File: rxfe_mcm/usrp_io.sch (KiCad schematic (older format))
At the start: 24 parts, among them J201 DB15, P201 CONN_02X10, U202 CONN_SMA, U203 74HC04_FULL, U204 CONN_SMA, U205 ADP7158, U206 CONN_SMA, U209 CONN_SMA

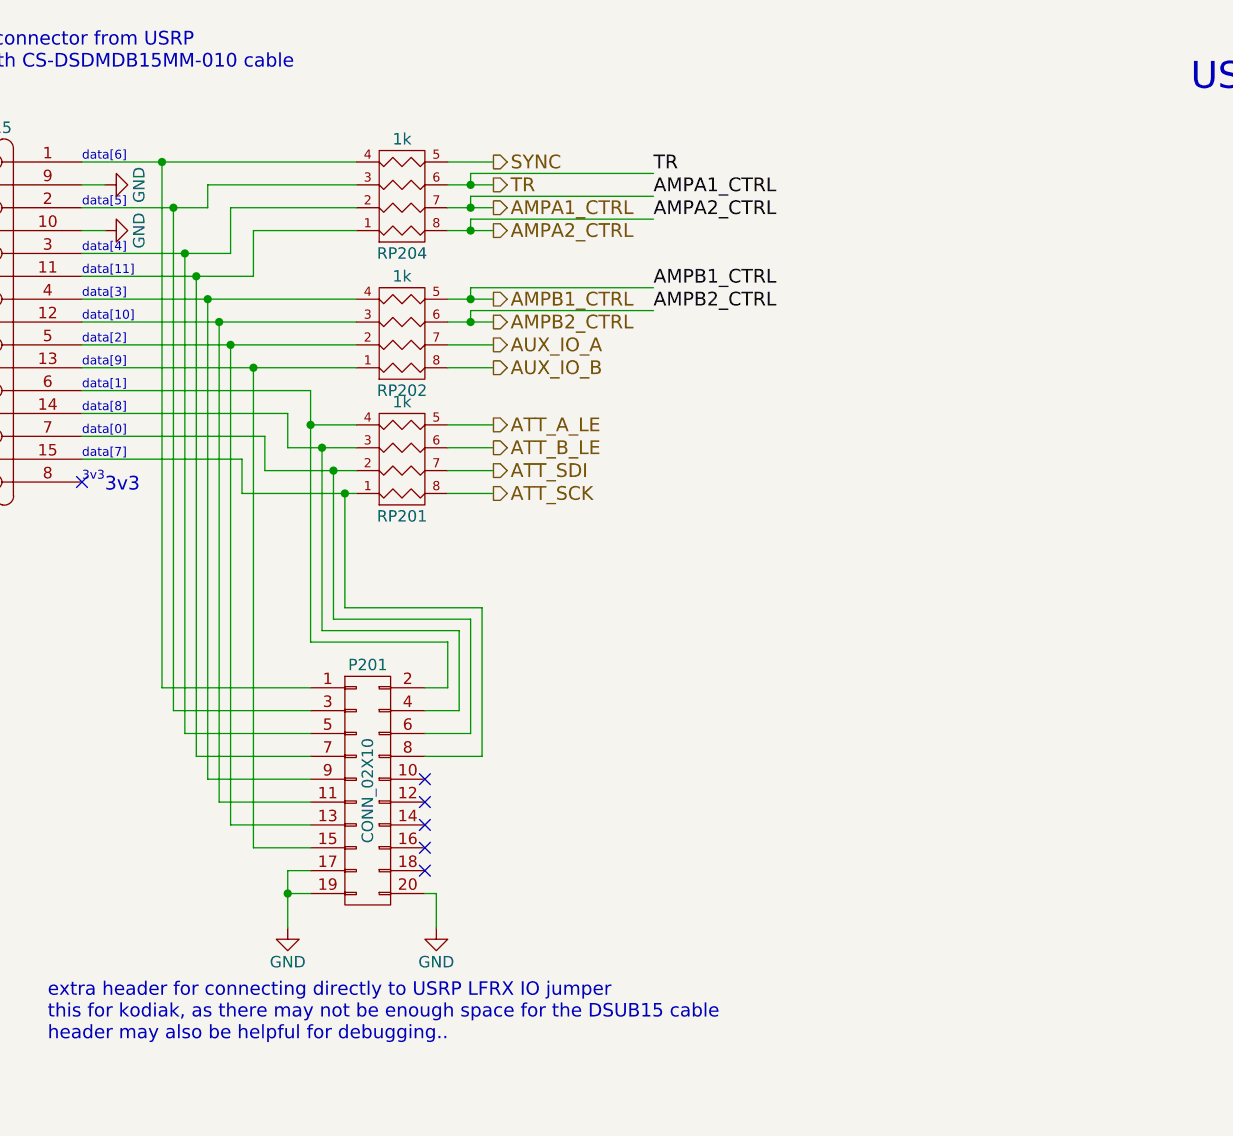
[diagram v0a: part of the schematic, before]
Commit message: a bit of work on layout..
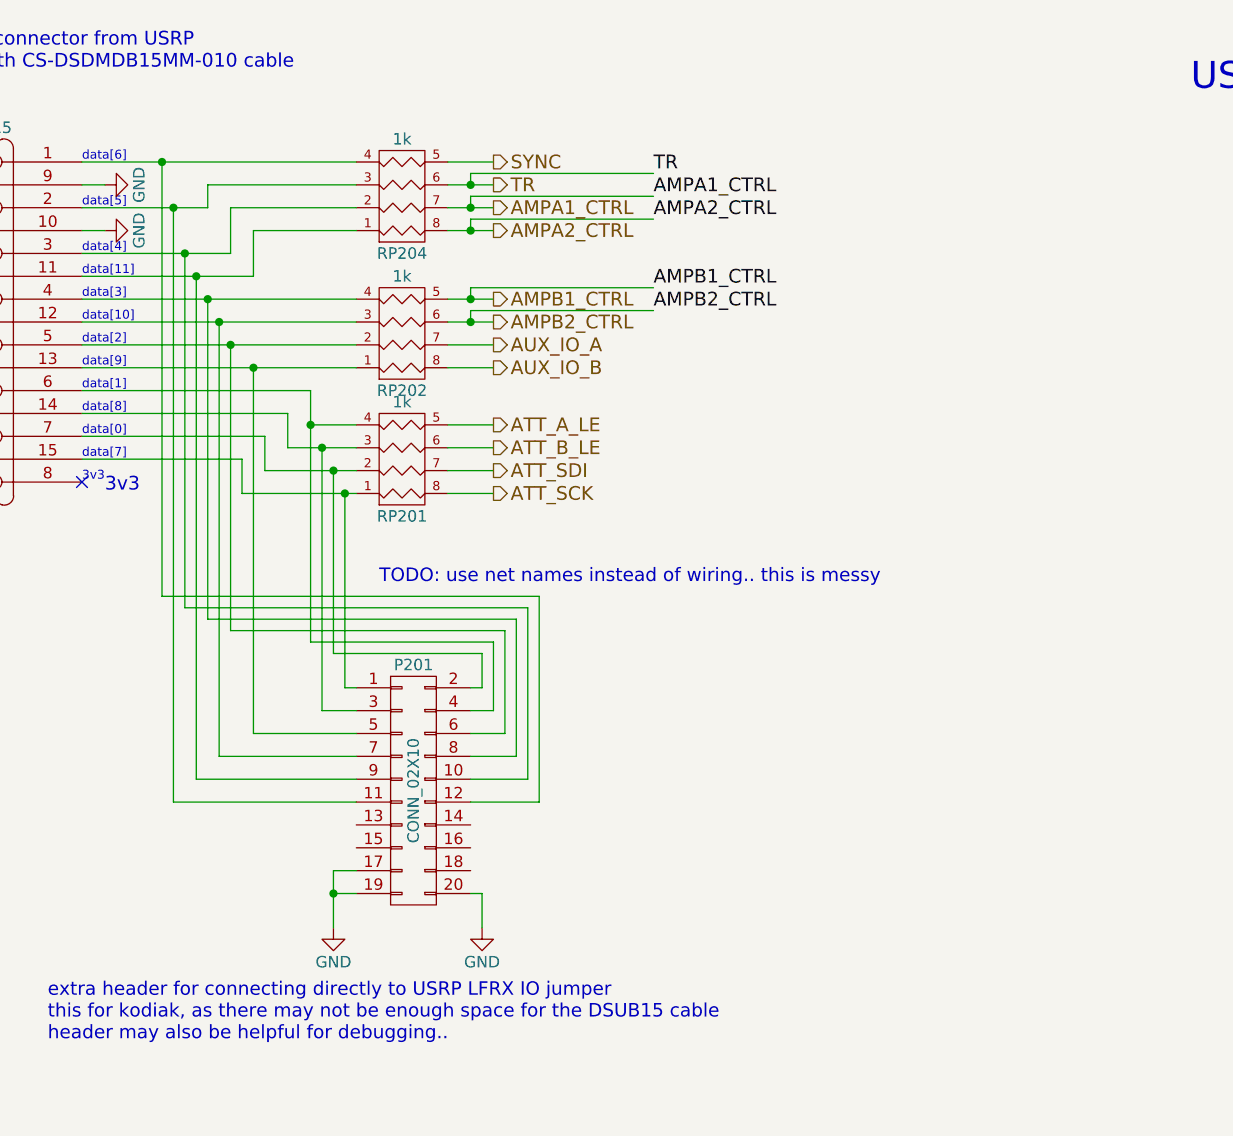
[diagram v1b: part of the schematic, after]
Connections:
- net at J201.1, RP204.4 (P4): now also P201.12 (P12); no longer P201.1 (P1)
- net at J201.11 (P111), RP204.1 (P1): now also P201.9 (P9); no longer P201.7 (P7)
- net at J201.12 (P12), RP202.3 (P3): now also P201.7 (P7); no longer P201.11 (P11)
- net at J201.13 (P13), RP202.1 (P1): now also P201.5 (P5); no longer P201.15 (P15)
- net at J201.14 (P14), RP201.3 (P3): now also P201.3 (P3); no longer P201.4 (P4)
- net at J201.15 (P15), RP201.1 (P1): now also P201.1 (P1); no longer P201.8 (P8)
- net at J201.2, RP204.3 (P3): now also P201.11 (P11); no longer P201.3 (P3)
- net at J201.3, RP204.2 (P2): now also P201.10 (P10); no longer P201.5 (P5)
- net at J201.4, RP202.4 (P4): now also P201.8 (P8); no longer P201.9 (P9)
- net at J201.5, RP202.2 (P2): now also P201.6 (P6); no longer P201.13 (P13)
- net at J201.6, RP201.4 (P4): now also P201.4 (P4); no longer P201.2 (P2)
- net at J201.7, RP201.2 (P2): now also P201.2 (P2); no longer P201.6 (P6)
- no-connect marks 6 -> 1
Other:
- note added: "TODO: use net names instead of wiring.. this is messy"
- moved on the sheet: P201
